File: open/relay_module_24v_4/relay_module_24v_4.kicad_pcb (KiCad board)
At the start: 2 copper layers, 67.6 x 77.1 mm, 22 parts, among them J1 Conn_01x12_Pin, J4 Conn_01x05_Pin, K1 Relay_SPDT, K2 Relay_SPDT, K3 Relay_SPDT, K4 Relay_SPDT

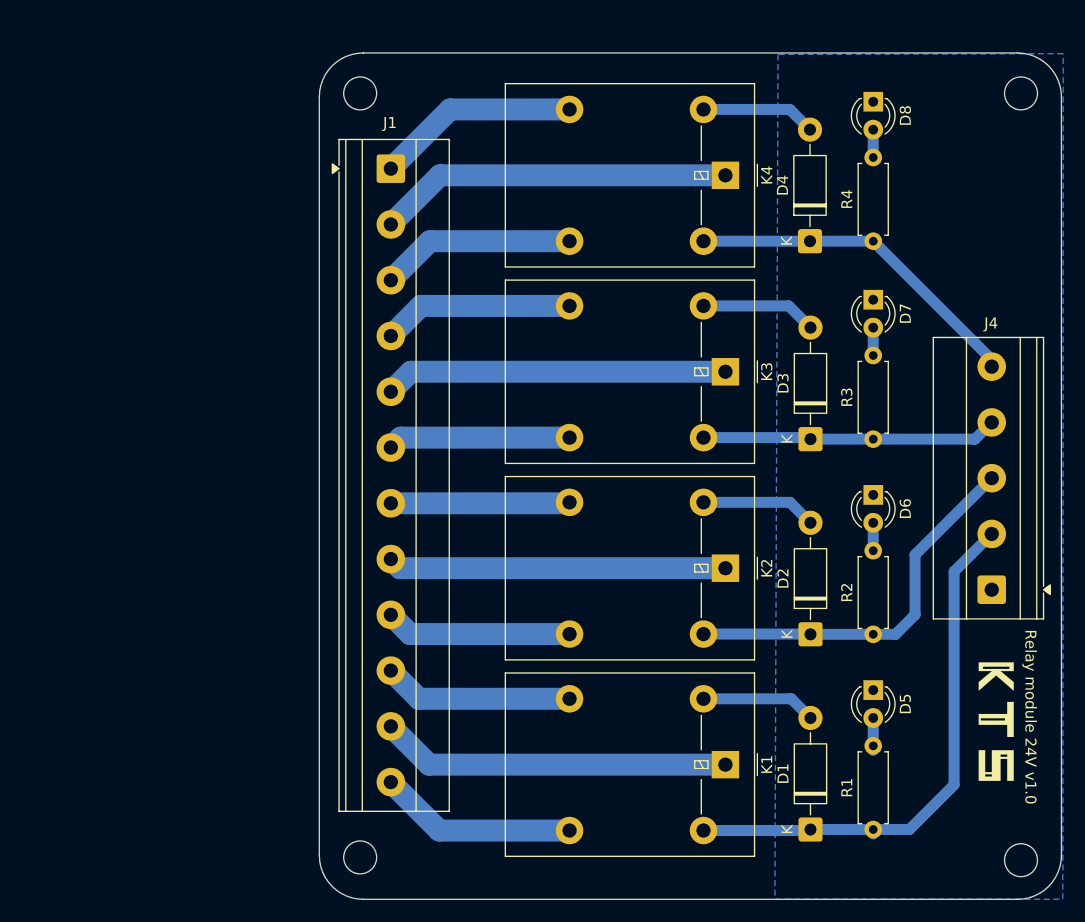
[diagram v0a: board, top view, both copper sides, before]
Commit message: v1.0.0
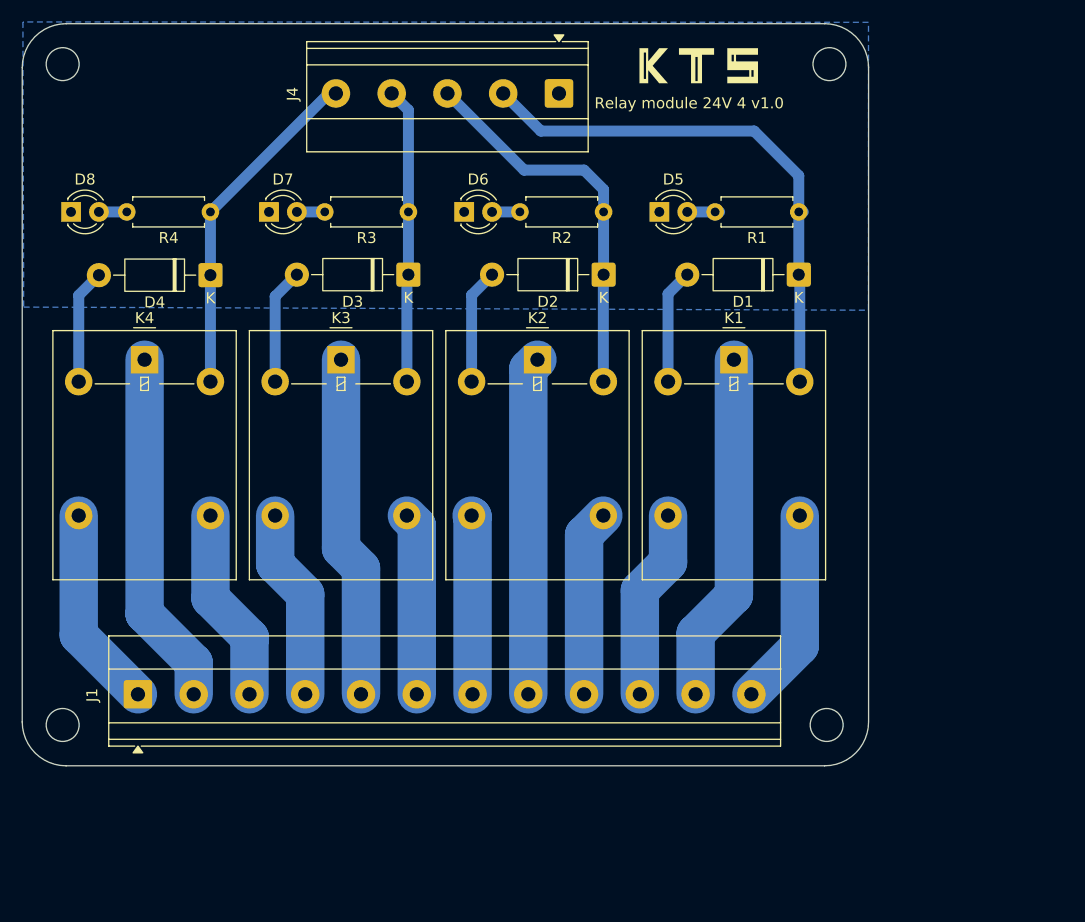
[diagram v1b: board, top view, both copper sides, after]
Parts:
- removed the REF** at (184.7, 141.0)
- removed the REF** at (124.5, 71.1)
- removed the REF** at (184.7, 71.1)
- removed the REF** at (124.5, 140.7)
- added REF**: MH_3mm, MountingHole:MountingHole_3mm, F.Cu at (167.0, 128.7)
- added REF**: MH_3mm, MountingHole:MountingHole_3mm, F.Cu at (97.4, 128.7)
- added REF**: MH_3mm, MountingHole:MountingHole_3mm, F.Cu at (167.2, 68.5)
- added REF**: MH_3mm, MountingHole:MountingHole_3mm, F.Cu at (97.4, 68.5)
- moved D8 73.8 mm to (98.1, 81.9), turned to 0 degrees
- moved R4 60.4 mm to (110.8, 81.9), turned to 180 degrees
- moved J4 60.0 mm to (142.6, 71.1), turned to 180 degrees
- moved R1 56.7 mm to (164.4, 81.9), turned to 180 degrees
- moved D7 55.6 mm to (116.2, 81.9), turned to 0 degrees
- moved K4 55.5 mm to (104.8, 95.4), turned to 0 degrees
- moved D4 54.7 mm to (110.8, 87.7), turned to 180 degrees
- moved J1 53.1 mm to (104.2, 125.9), turned to 0 degrees
- moved D1 50.6 mm to (164.4, 87.6), turned to 180 degrees
- moved D5 47.7 mm to (151.7, 81.9), turned to 0 degrees
- moved R3 47.1 mm to (128.9, 81.9), turned to 180 degrees
- moved R2 45.7 mm to (146.6, 81.9), turned to 180 degrees
- moved D6 45.3 mm to (133.9, 81.9), turned to 0 degrees
- moved D3 39.6 mm to (128.9, 87.6), turned to 180 degrees
- moved D2 37.8 mm to (146.6, 87.6), turned to 180 degrees
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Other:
- board size 67.6 x 77.1 mm -> 77.1 x 67.6 mm
- board text added: "Relay module 24V 4 v1.0"
- board text removed: "Relay module 24V v1.0"
